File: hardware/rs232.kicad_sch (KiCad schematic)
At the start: 1 part, among them U5 MAX232N

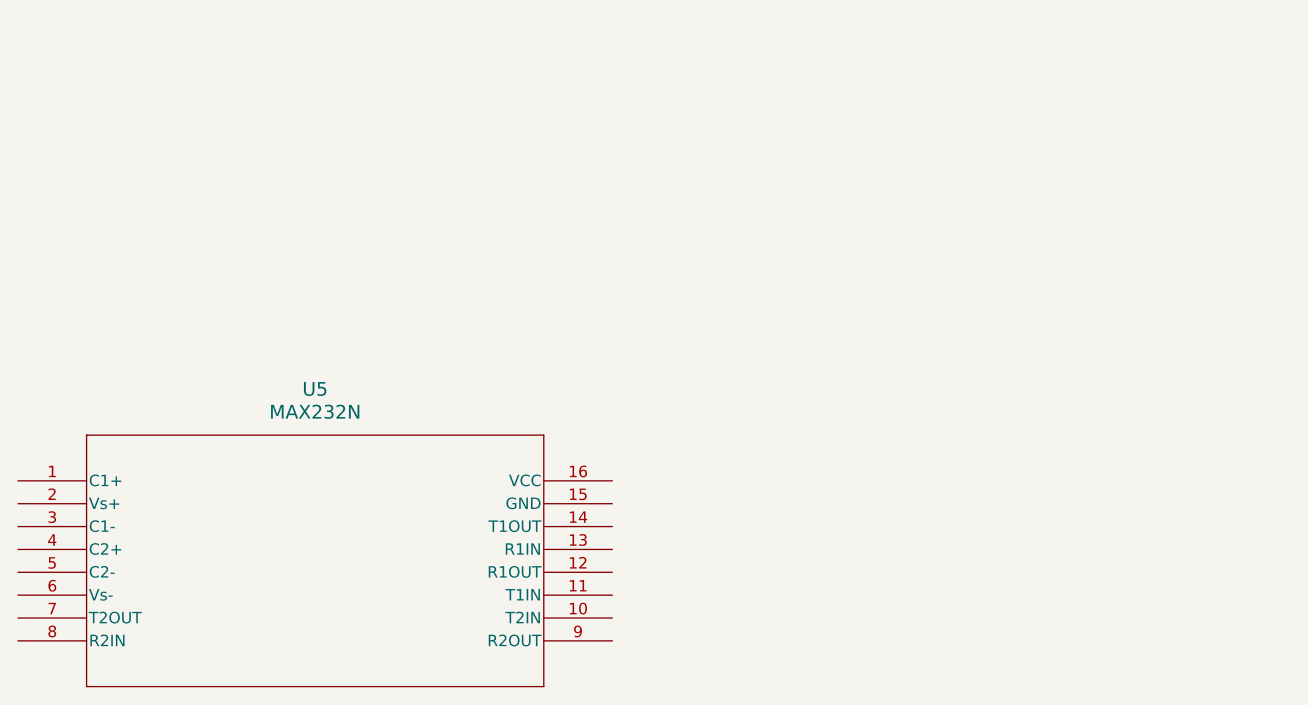
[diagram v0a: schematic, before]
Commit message: Kicad şema düzenlemesi yapıldı.
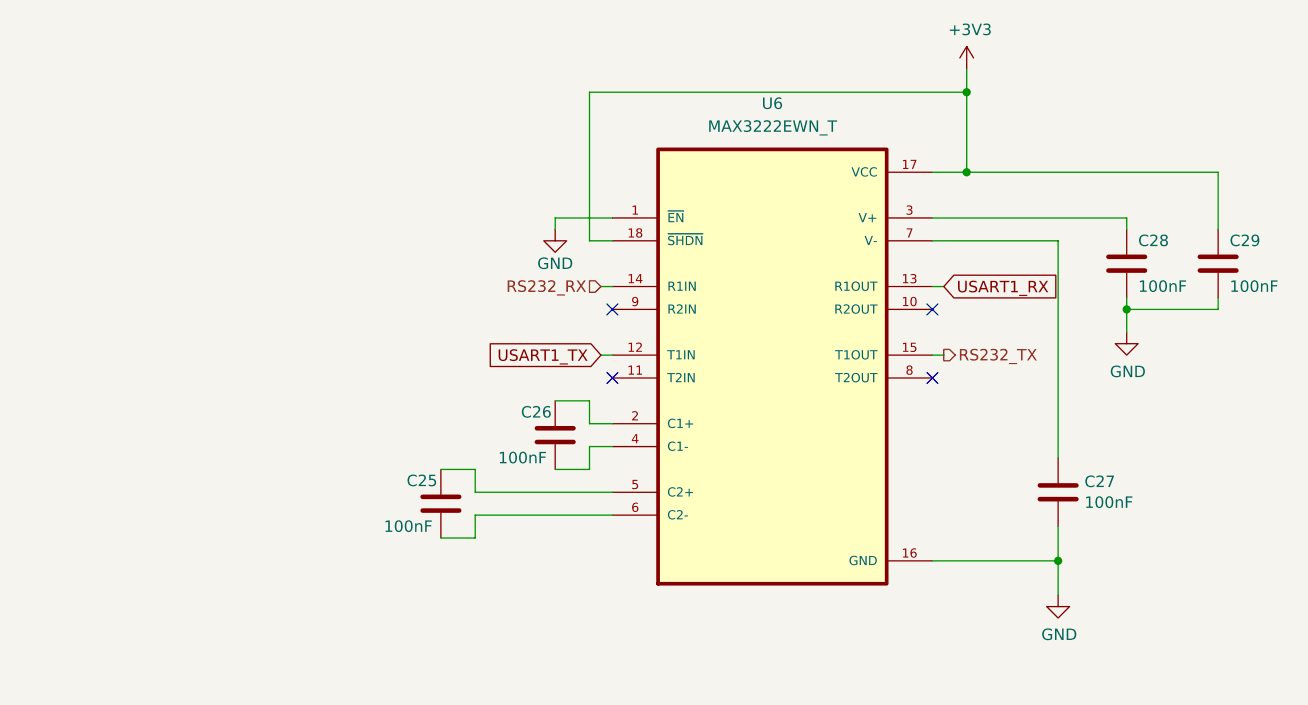
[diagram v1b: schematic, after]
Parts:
- removed U5: MAX232N, N16, symbol drip-irrigation-sys-cc:MAX232N
- added C25, C26, C27, C28, C29: 100nF, Capacitor_SMD:C_0603_1608Metric, symbol Device:C
- added U6: MAX3222EWN_T, MAX3222EWN_T:SOIC127P1032X265-18N, symbol drip-irrigation-sys-cc:MAX3222EWN_T
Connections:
- new net: C28.1, U6.3 (V+)
- new net: C27.1, U6.7 (V-)
- new net: C26.1, U6.2 (C1+)
- new net: C26.2, U6.4 (C1-)
- new net: C25.1, U6.5 (C2+)
- new net: C25.2, U6.6 (C2-)
- new net +3V3: C29.1, U6.17 (VCC), U6.18 (~{SHDN})
- new net GND: C27.2, C28.2, C29.2, U6.1 (~{EN}), U6.16 (GND)
- new net RS232_RX: U6.14 (R1IN)
- new net RS232_TX: U6.15 (T1OUT)
- new net USART1_RX: U6.13 (R1OUT)
- new net USART1_TX: U6.12 (T1IN)
- no-connect marks 0 -> 4
